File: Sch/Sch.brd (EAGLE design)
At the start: 100 x 100 mm, 85 parts, among them IC1 MEGA8-P, IC10 MCP2221A, IC11 DIP-SW, IC2 74HC595N, IC3 YMZ294, IC4 YMZ294, IC5 YMZ294, IC6 YM2413, IC7 TLP2630, IC8 NJM2114, IC9 SSM2019, Q1 16MHz, T1 2SA1015, T2 2SD468

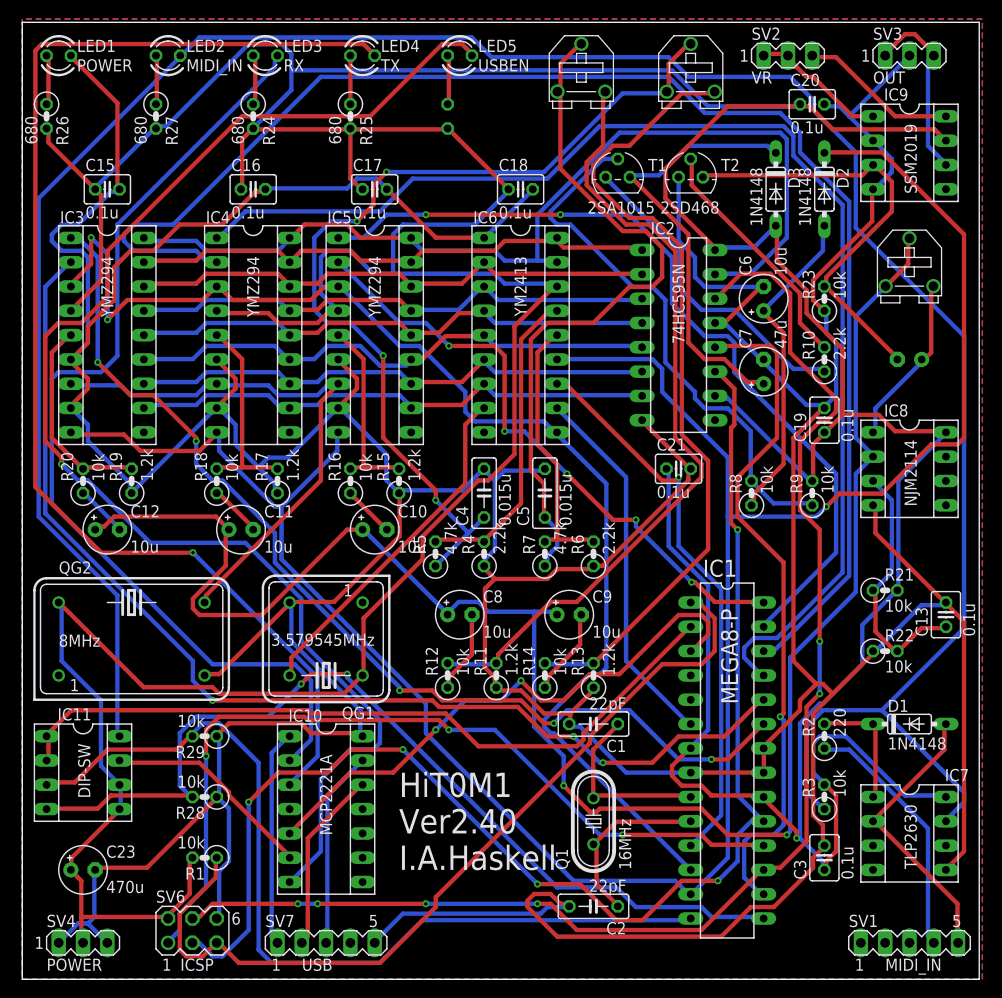
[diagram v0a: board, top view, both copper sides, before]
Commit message: Update Readme.md
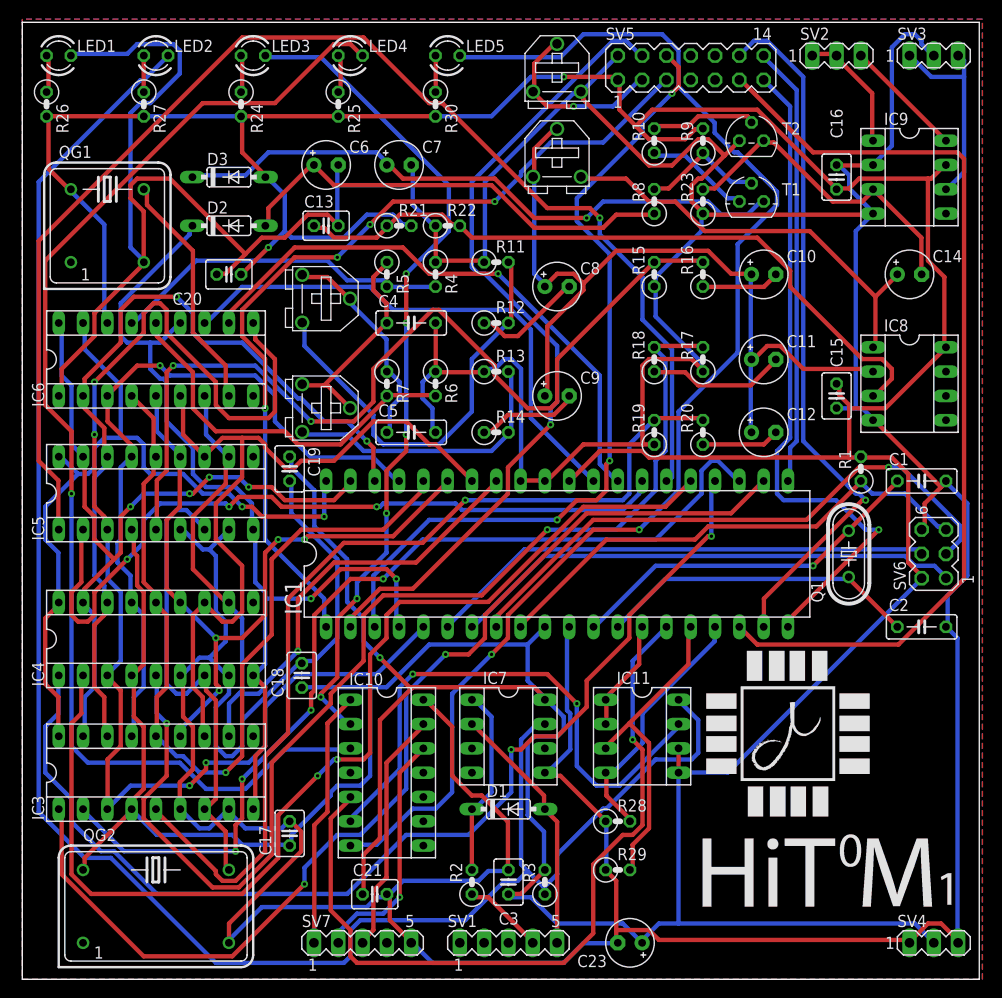
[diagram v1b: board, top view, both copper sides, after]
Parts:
- removed IC2: 74HC595N, 74xx-eu:DIL16
- added SV5: LCD, con-lstb:MA07-2
- added VR4: TSR-065, akizuki:TSR-065
- IC1: value MEGA8-P -> MEGA32-P; device atmel:DIL28-3 -> atmel:DIL40
- moved SV4 88.9 mm to (95.2, 3.81)
- moved SV6 86.9 mm to (95.2, 44.5), turned to 90 degrees
- moved R1 79.7 mm to (87.6, 53.3), turned to 90 degrees
- moved C15 79.2 mm to (85.1, 61.0), turned to 270 degrees
- moved C13 76.5 mm to (31.8, 78.7), turned to 0 degrees
- moved C12 69.3 mm to (77.5, 57.1)
- moved C17 67.9 mm to (27.9, 15.2), turned to 90 degrees
- moved R20 65.0 mm to (71.1, 57.1)
- moved R22 63.8 mm to (44.5, 78.7)
- moved C20 63.5 mm to (21.6, 73.7), turned to 180 degrees
- moved R21 63.5 mm to (39.4, 78.7)
- moved D2 62.3 mm to (21.6, 78.7), turned to 0 degrees
- moved C16 61.0 mm to (85.1, 83.8), turned to 90 degrees
- moved IC11 58.5 mm to (64.8, 25.4)
- moved C23 57.7 mm to (63.5, 3.81), turned to 180 degrees
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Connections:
- removed net N$3: C1.1, IC1.9, Q1.2
- removed net RCK: IC1.16, IC2.12
- new net DB4: IC1.18, SV5.11
- new net DB5: IC1.19, SV5.12
- new net DB6: IC1.20, SV5.13
- new net DB7: IC1.21, SV5.14
- new net E: IC1.3, SV5.6
- new net N$28: C1.1, IC1.12, Q1.2
- new net N$38: SV5.8
- new net N$39: SV5.10
- new net N$44: SV5.7
- new net N$45: SV5.9
- new net R/W: IC1.1, SV5.5
- new net RS: IC1.2, SV5.4
- new net VO: SV5.3, VR4.1, VR4.2
- net A0: now also IC1.5; no longer IC1.12
- net CONFIG1: now also IC1.16; no longer IC1.14
- net CONFIG2: now also IC1.17; no longer IC1.15
- net DATA0: now also IC1.40; no longer IC2.15
- net DATA1: now also IC1.39; no longer IC2.1
- net DATA2: now also IC1.38; no longer IC2.2
- net DATA3: now also IC1.37; no longer IC2.3
- net DATA4: now also IC1.36; no longer IC2.4
- net DATA5: now also IC1.35; no longer IC2.5
- net DATA6: now also IC1.34; no longer IC2.6
- net DATA7: now also IC1.33; no longer IC2.7
- net FM_CS: now also IC1.29; no longer IC1.11
- net FM_WE: now also IC1.28; no longer IC1.6
- net GND: now also IC1.11, IC1.31, IC1.32, SV5.2, VR4.3; no longer IC1.21, IC1.22, IC1.8, IC2.13, IC2.8
- net IC: now also IC1.4; no longer IC1.13
- net MISO: now also IC1.7; no longer IC1.18
- net MOSI: now also IC1.6; no longer IC1.17, IC2.14
- net N$4: now also IC1.13; no longer IC1.10
- net PSG1_CS: now also IC1.23; no longer IC1.24
- net PSG1_WR: now also IC1.22; no longer IC1.23
- net PSG2_CS: now also IC1.25; no longer IC1.26
- net PSG2_WR: now also IC1.24; no longer IC1.25
- net PSG3_CS: now also IC1.27; no longer IC1.28
- net PSG3_WR: now also IC1.26; no longer IC1.27
- net RST: now also IC1.9; no longer IC1.1
- net RX: now also IC1.14; no longer IC1.2
- net SCK: now also IC1.8; no longer IC1.19, IC2.11
- net TX: now also IC1.15; no longer IC1.3
- net VCC: now also IC1.10, IC1.30, SV5.1; no longer IC1.20, IC1.7, IC2.10, IC2.16
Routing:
- net IC: track 241.0 -> 100.1 mm, vias 1 -> 2
- net PSG2_OUT: track 21.4 -> 120.1 mm, vias 0 -> 2
- net N$10: track 186.3 -> 87.7 mm, vias 2 -> 0
- net DB4: track 0.00 -> 97.9 mm
- net R/W: track 0.00 -> 91.2 mm, vias 0 -> 4
- net MOSI: track 142.3 -> 53.2 mm, vias 6 -> 0
- net RS: track 0.00 -> 86.1 mm, vias 0 -> 1
- net E: track 0.00 -> 85.4 mm, vias 0 -> 3
- net SCK: track 140.4 -> 62.1 mm, vias 5 -> 1
- net PSG1_OUT: track 21.5 -> 97.8 mm, vias 0 -> 1
- net PSG3_OUT: track 20.2 -> 96.4 mm, vias 0 -> 2
- net N$8: track 96.7 -> 22.8 mm, vias 4 -> 0
- net DB5: track 0.00 -> 73.9 mm, vias 0 -> 1
- net RCK: track 71.5 -> 0.00 mm, vias 1 -> 0
- net DB6: track 0.00 -> 71.2 mm, vias 0 -> 1
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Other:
- board text added: "C:/Users/Ivory/Desktop/idesa.bmp"
- board text removed: "HiT0M1 Ver2.40 I.A.Haskell"
